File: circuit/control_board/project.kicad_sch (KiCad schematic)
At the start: 0 parts

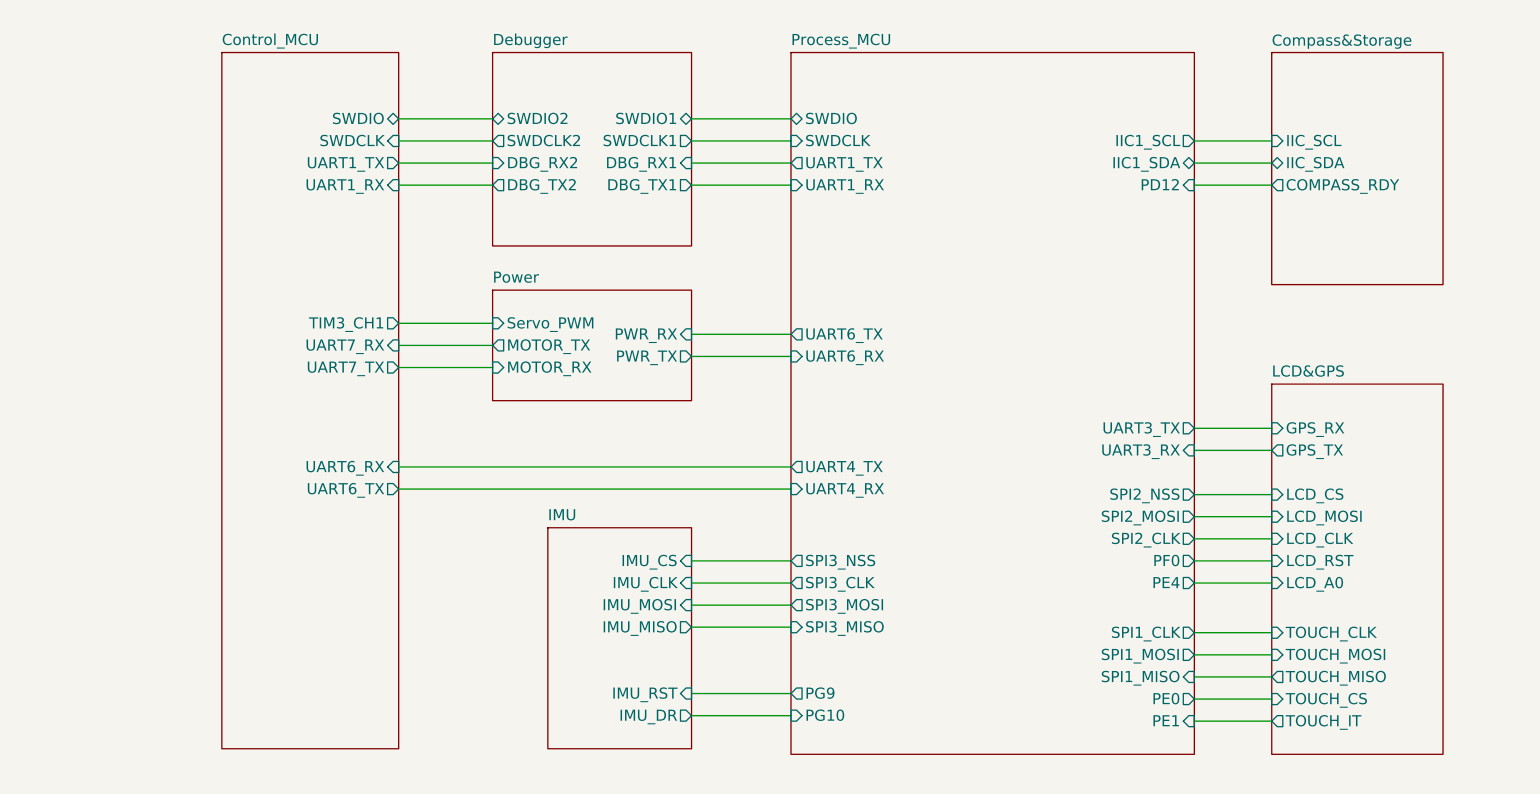
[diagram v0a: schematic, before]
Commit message: Modified the circuitry of the main control board to add a microcontroller for reading information from the magnetometer and IMU. Modified the SPI connection port of the Process MCU.
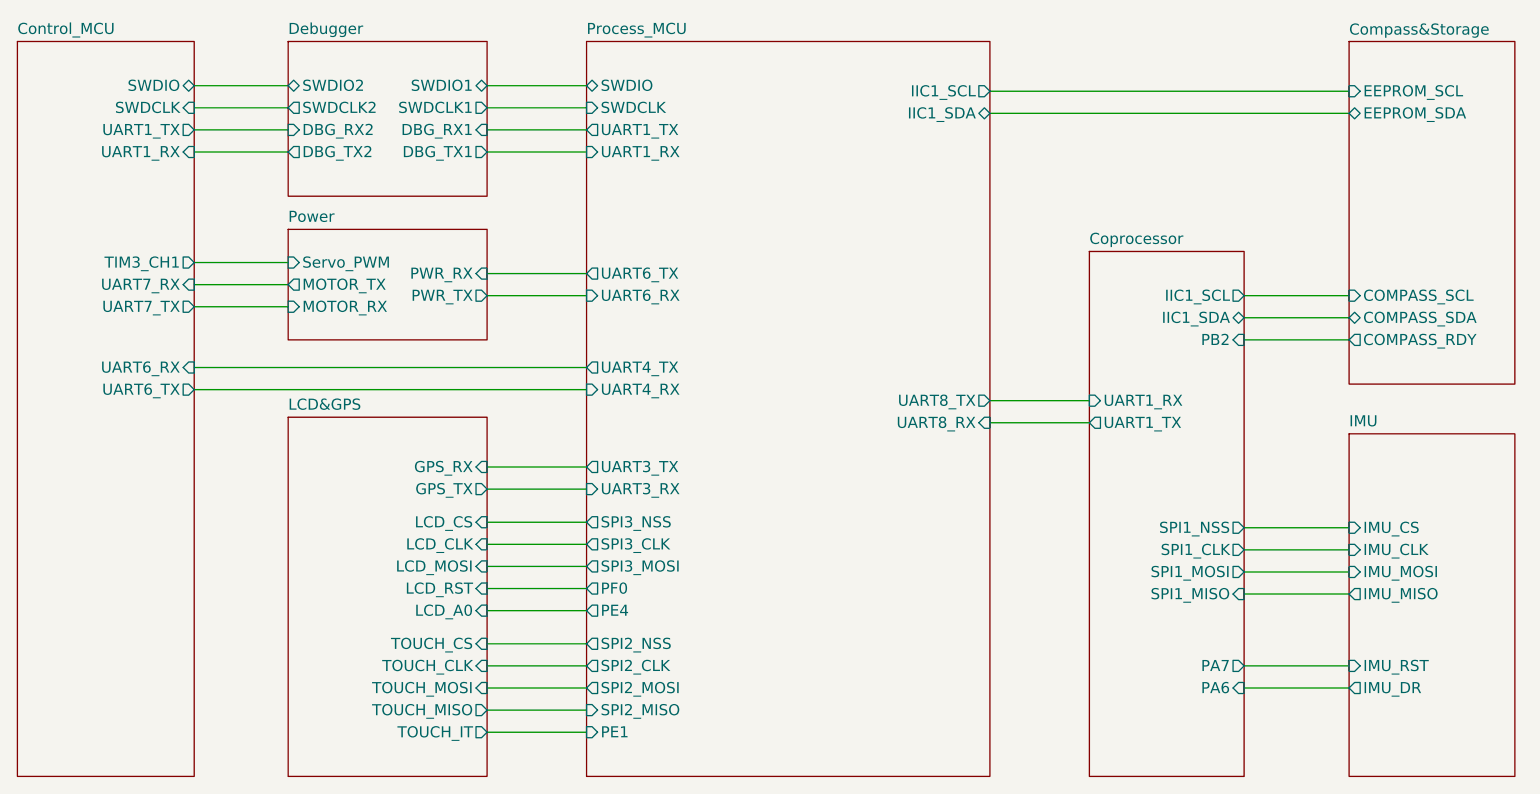
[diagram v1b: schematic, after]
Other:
- added sheet Coprocessor (Coprocessor.kicad_sch)
- sheet Compass&Storage ports: added COMPASS_SCL, COMPASS_SDA, EEPROM_SCL, EEPROM_SDA; removed IIC_SCL, IIC_SDA
- sheet Process_MCU ports: added SPI2_MISO, UART8_RX, UART8_TX; removed PD12, PE0, PG10, PG9, SPI1_CLK, SPI1_MISO, SPI1_MOSI, SPI3_MISO
